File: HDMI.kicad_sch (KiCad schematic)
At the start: 2 parts, among them J1 HDMI_A, J2 HDMI_A

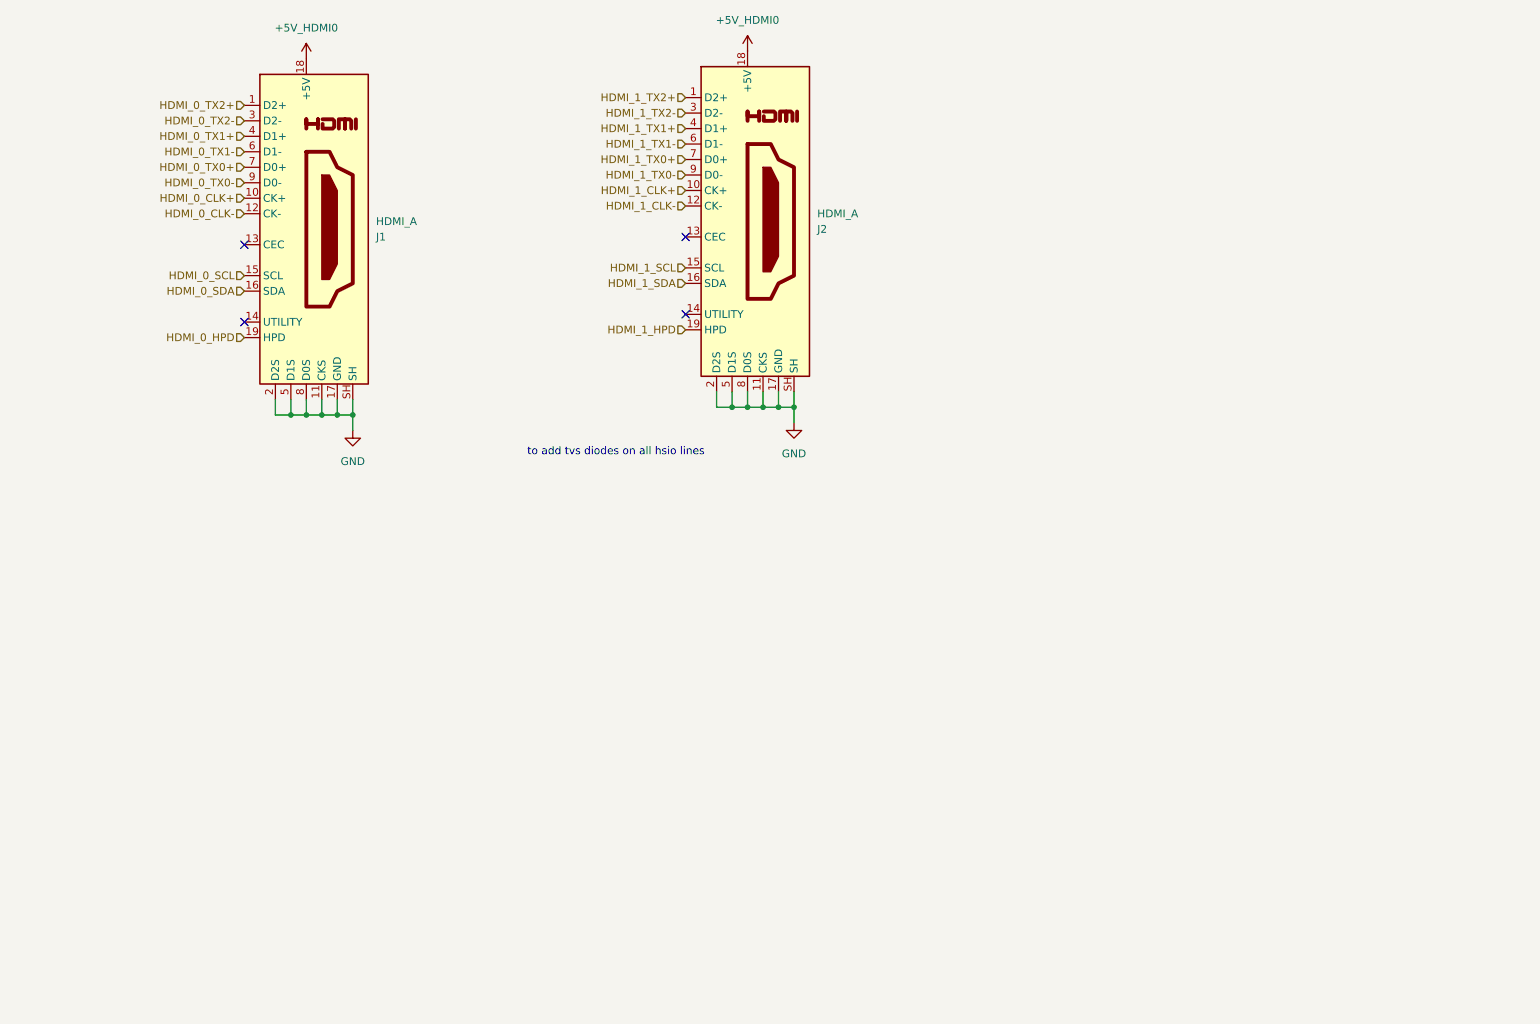
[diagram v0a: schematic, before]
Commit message: .
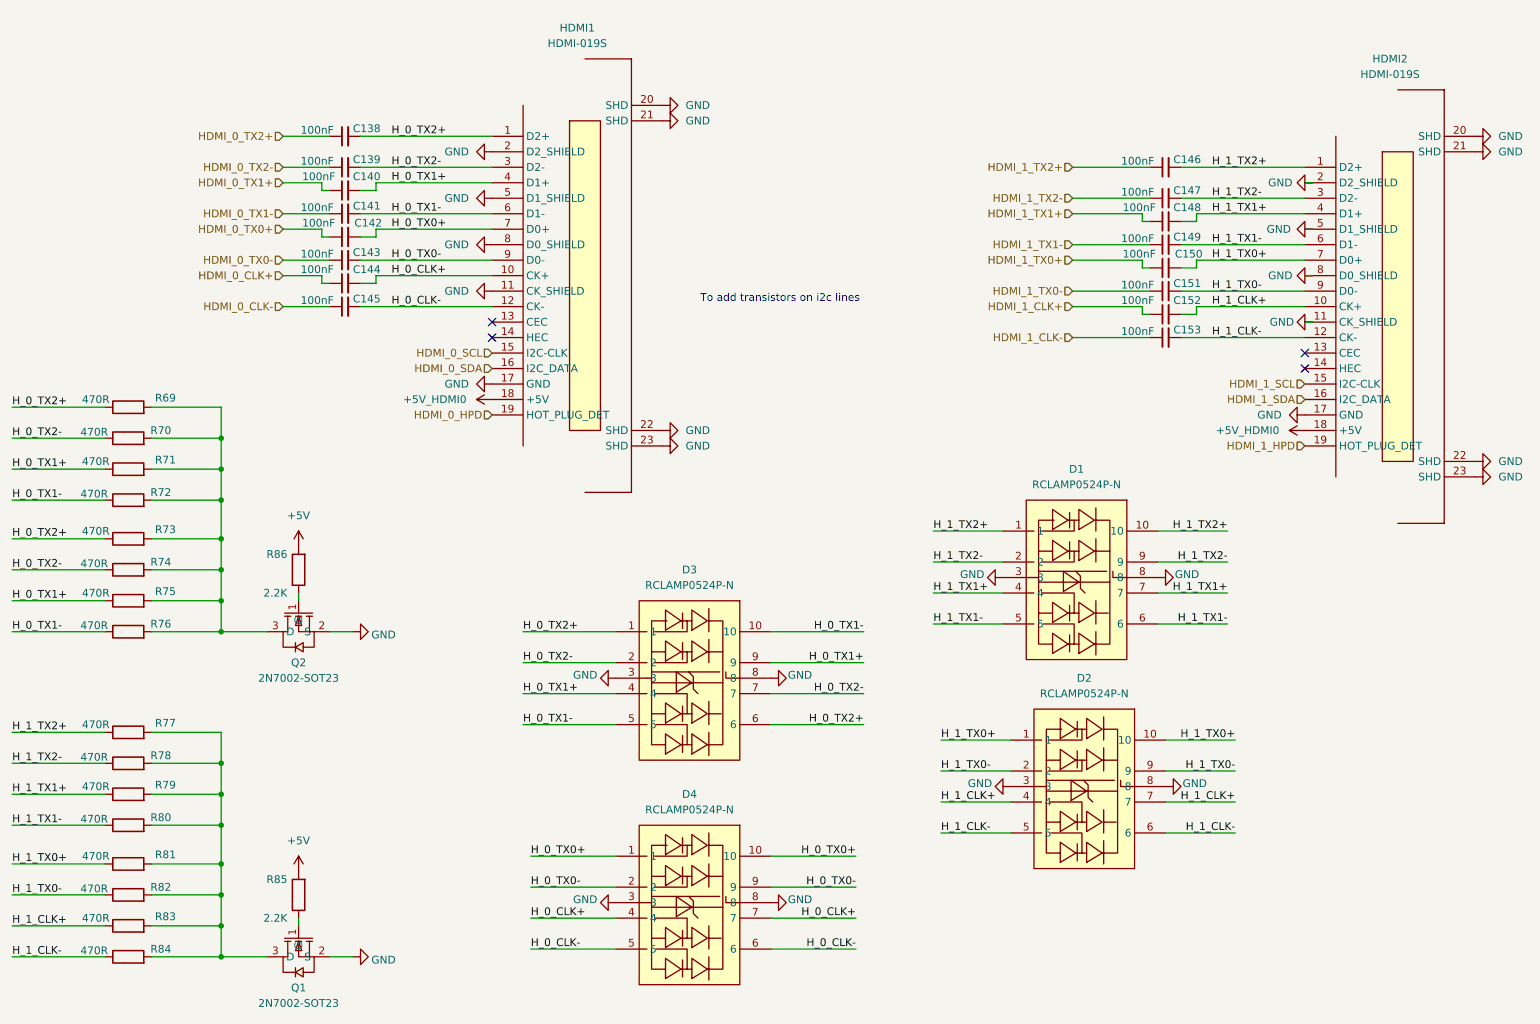
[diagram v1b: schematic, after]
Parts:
- removed J1, J2: HDMI_A, symbol Connector:HDMI_A
- added C138, C139, C140, C141, C142, C143, C144, C145, C146, C147, C148, C149, C150, C151, C152, C153: 100nF, Capacitor_SMD:C_0402_1005Metric, symbol Device:C_Small
- added D1, D2, D3, D4: RCLAMP0524P-N, easyeda2kicad:DFN-10L_L2.5-W1.0-P0.50-BL, symbol da:RCLAMP0524P-N
- added HDMI1, HDMI2: HDMI-019S, easyeda2kicad:HDMI-SMD_HDMI-019S, symbol da:HDMI-019S
- added Q1, Q2: 2N7002-SOT23, easyeda2kicad:SOT-23_L2.9-W1.3-P1.90-LS2.4-BR, symbol da:2N7002-SOT23
- added R69, R70, R71, R72, R73, R74, R75, R76, R77, R78, R79, R80, R81, R82, R83, R84: 470R, Resistor_SMD:R_0402_1005Metric, symbol Device:R
- added R85, R86: 2.2K, Resistor_SMD:R_0402_1005Metric, symbol Device:R
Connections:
- net +5V_HDMI0: now also HDMI1.18 (+5V), HDMI2.18 (+5V)
- net GND: now also D1.3, D1.8, D2.3, D2.8, D3.3, D3.8, D4.3, D4.8, HDMI1.11 (CK_SHIELD), HDMI1.17 (GND), HDMI1.2 (D2_SHIELD), HDMI1.20 (SHD), HDMI1.21 (SHD), HDMI1.22 (SHD), HDMI1.23 (SHD), HDMI1.5 (D1_SHIELD), HDMI1.8 (D0_SHIELD), HDMI2.11 (CK_SHIELD), HDMI2.17 (GND), HDMI2.2 (D2_SHIELD), HDMI2.20 (SHD), HDMI2.21 (SHD), HDMI2.22 (SHD), HDMI2.23 (SHD), HDMI2.5 (D1_SHIELD), HDMI2.8 (D0_SHIELD), Q1.2 (S), Q2.2 (S)
- net HDMI_0_CLK+: now also C144.1
- net HDMI_0_CLK-: now also C145.1
- net HDMI_0_HPD: now also HDMI1.19 (HOT_PLUG_DET)
- net HDMI_0_SCL: now also HDMI1.15 (I2C-CLK)
- net HDMI_0_SDA: now also HDMI1.16 (I2C_DATA)
- net HDMI_0_TX0+: now also C142.1
- net HDMI_0_TX0-: now also C143.1
- net HDMI_0_TX1+: now also C140.1
- net HDMI_0_TX1-: now also C141.1
- net HDMI_0_TX2+: now also C138.1
- net HDMI_0_TX2-: now also C139.1
- net HDMI_1_CLK+: now also C152.1
- net HDMI_1_CLK-: now also C153.1
- net HDMI_1_HPD: now also HDMI2.19 (HOT_PLUG_DET)
- net HDMI_1_SCL: now also HDMI2.15 (I2C-CLK)
- net HDMI_1_SDA: now also HDMI2.16 (I2C_DATA)
- net HDMI_1_TX0+: now also C150.1
- net HDMI_1_TX0-: now also C151.1
- net HDMI_1_TX1+: now also C148.1
- net HDMI_1_TX1-: now also C149.1
- net HDMI_1_TX2+: now also C146.1
- net HDMI_1_TX2-: now also C147.1
- new net: Q2.1 (G), R86.1
- new net: Q2.3 (D), R69.2, R70.2, R71.2, R72.2, R73.2, R74.2, R75.2, R76.2
- new net: Q1.1 (G), R85.1
- new net: Q1.3 (D), R77.2, R78.2, R79.2, R80.2, R81.2, R82.2, R83.2, R84.2
- new net +5V: R85.2, R86.2
- new net H_0_CLK+: C144.2, D4.4, D4.7, HDMI1.10 (CK+)
- new net H_0_CLK-: C145.2, D4.5, D4.6, HDMI1.12 (CK-)
- new net H_0_TX0+: C142.2, D4.1, D4.10, HDMI1.7 (D0+)
- new net H_0_TX0-: C143.2, D4.2, D4.9, HDMI1.9 (D0-)
- new net H_0_TX1+: C140.2, D3.4, D3.9, HDMI1.4 (D1+), R71.1, R75.1
- new net H_0_TX1-: C141.2, D3.10, D3.5, HDMI1.6 (D1-), R72.1, R76.1
- new net H_0_TX2+: C138.2, D3.1, D3.6, HDMI1.1 (D2+), R69.1, R73.1
- new net H_0_TX2-: C139.2, D3.2, D3.7, HDMI1.3 (D2-), R70.1, R74.1
- new net H_1_CLK+: C152.2, D2.4, D2.7, HDMI2.10 (CK+), R83.1
- new net H_1_CLK-: C153.2, D2.5, D2.6, HDMI2.12 (CK-), R84.1
- new net H_1_TX0+: C150.2, D2.1, D2.10, HDMI2.7 (D0+), R81.1
- new net H_1_TX0-: C151.2, D2.2, D2.9, HDMI2.9 (D0-), R82.1
- new net H_1_TX1+: C148.2, D1.4, D1.7, HDMI2.4 (D1+), R79.1
- new net H_1_TX1-: C149.2, D1.5, D1.6, HDMI2.6 (D1-), R80.1
- new net H_1_TX2+: C146.2, D1.1, D1.10, HDMI2.1 (D2+), R77.1
- new net H_1_TX2-: C147.2, D1.2, D1.9, HDMI2.3 (D2-), R78.1
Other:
- note added: "To add transistors on i2c lines"
- note removed: "to add tvs diodes on all hsio lines"
